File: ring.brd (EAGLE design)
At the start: 174.9 x 190 mm, 36 parts

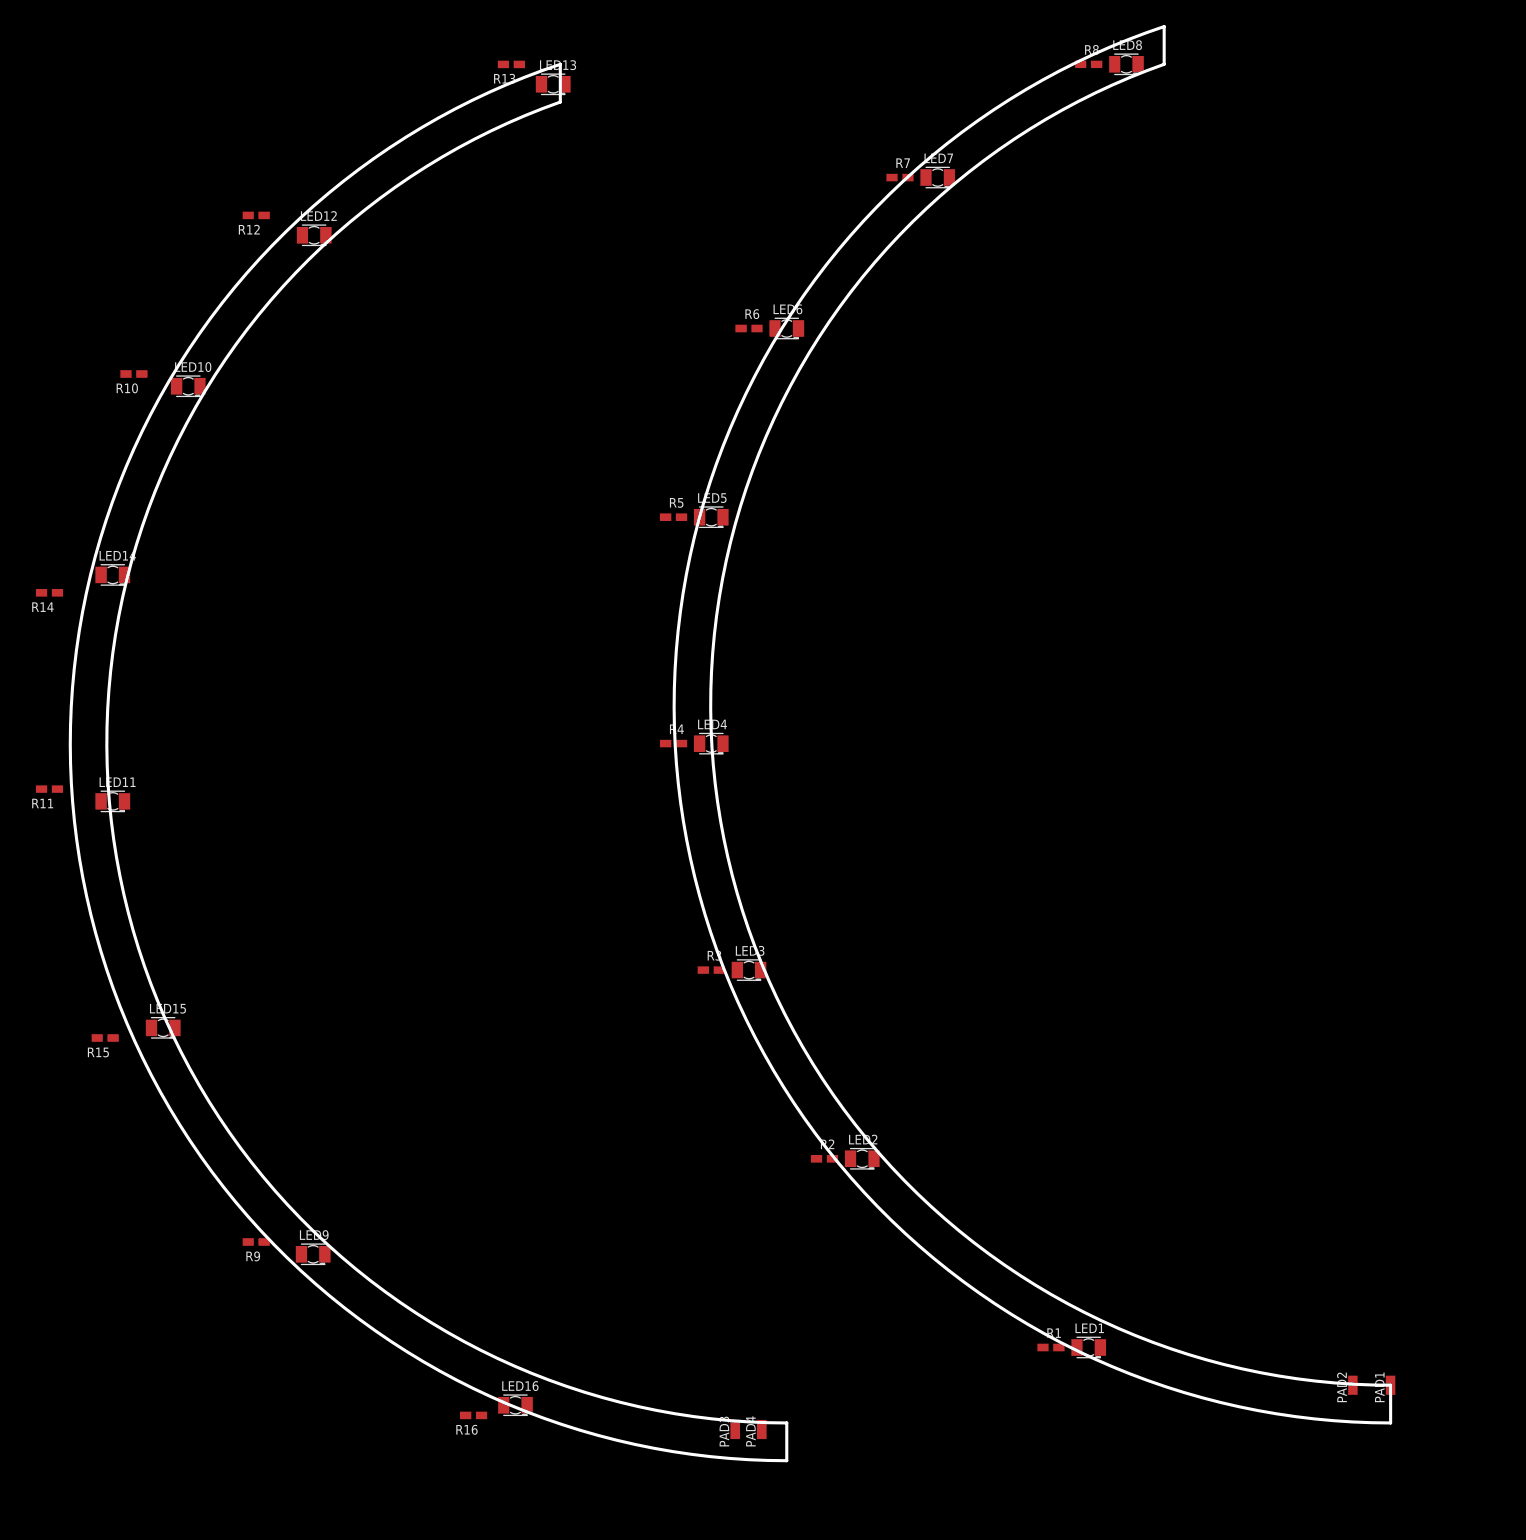
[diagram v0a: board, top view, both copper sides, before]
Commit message: polygon
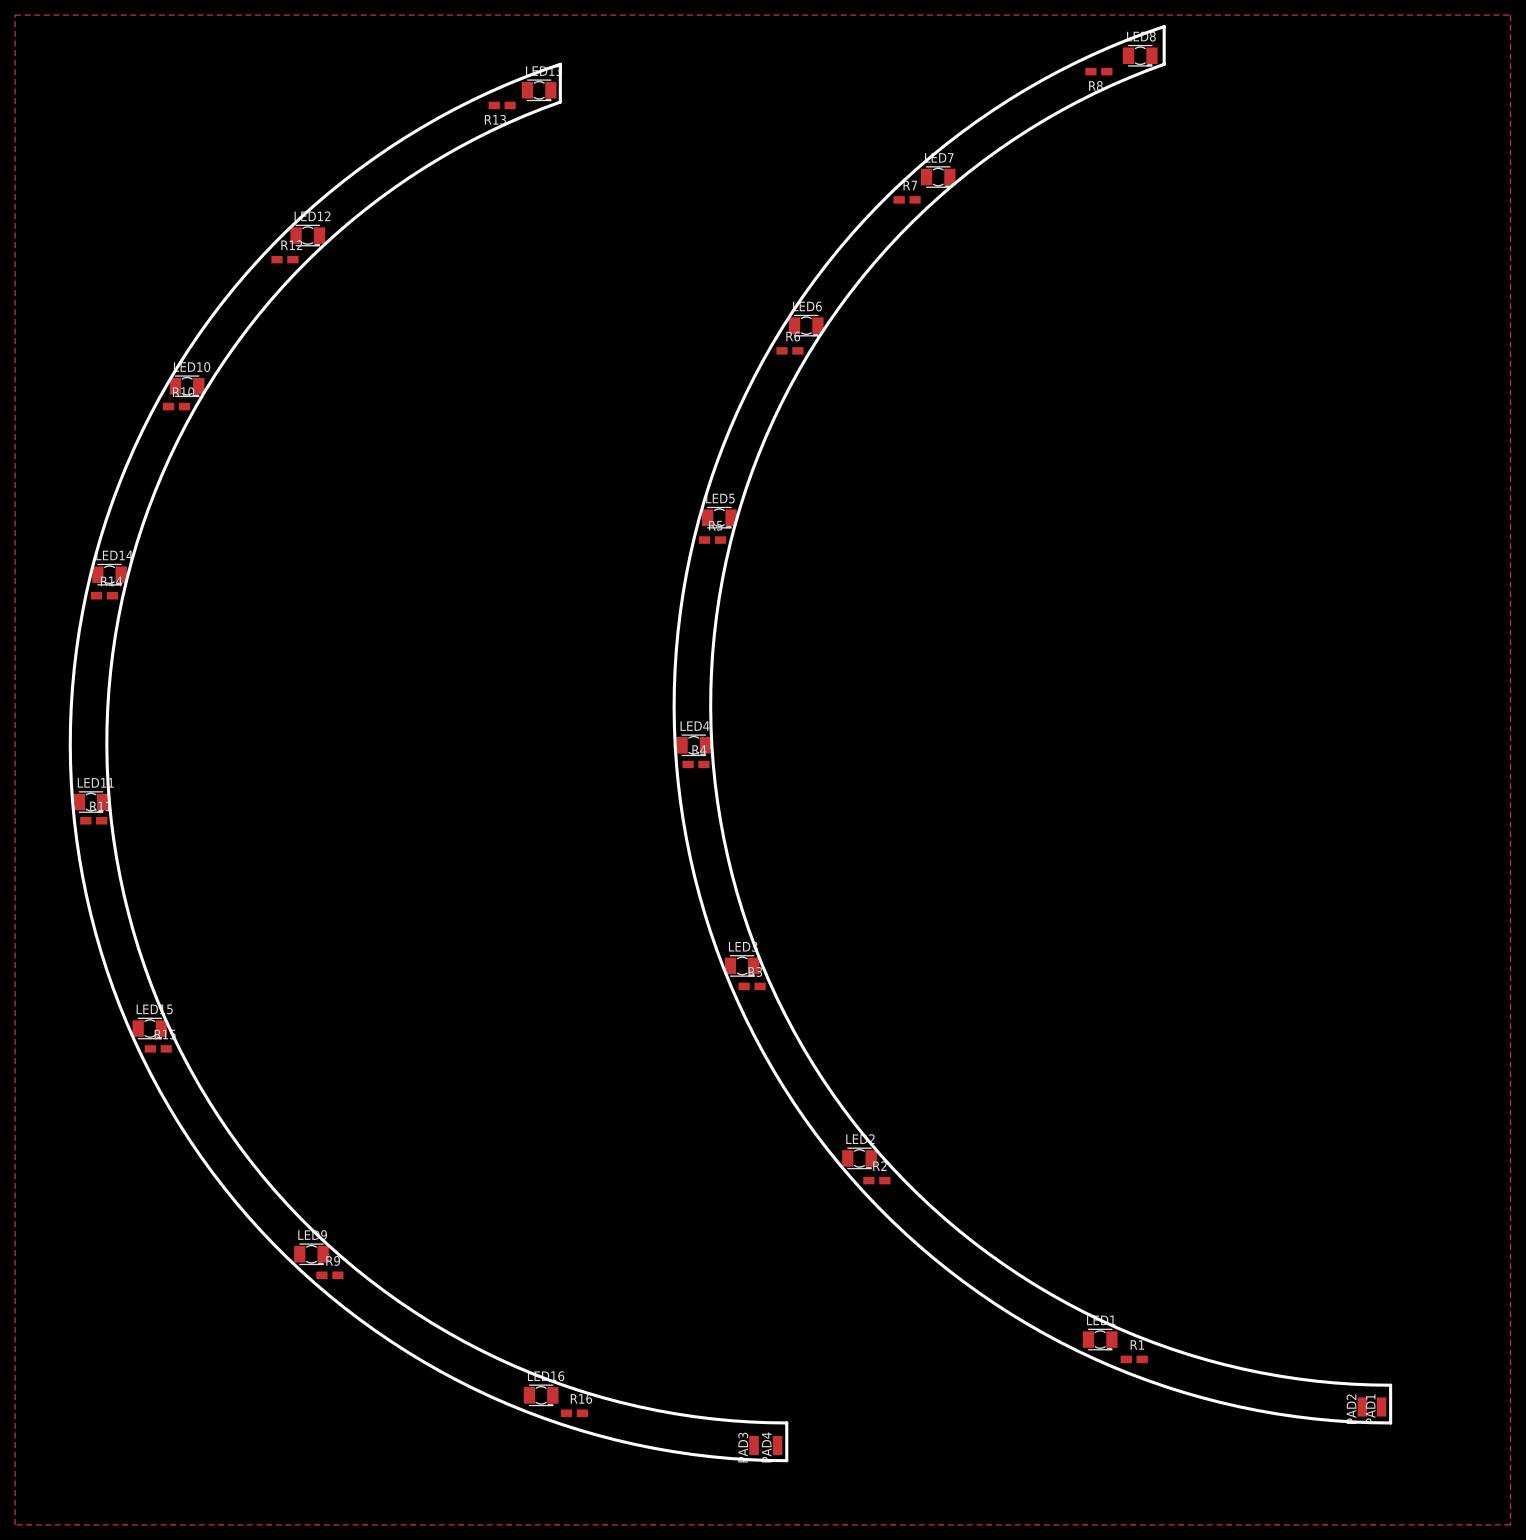
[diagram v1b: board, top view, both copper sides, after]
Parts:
- moved R16 13.4 mm to (-28.1, -88.7), turned to 0 degrees
- moved R1 11.1 mm to (46.0, -81.6)
- moved R9 10.7 mm to (-60.5, -70.4), turned to 0 degrees
- moved R2 7.52 mm to (11.9, -57.9)
- moved R14 7.29 mm to (-90.4, 19.6), turned to 0 degrees
- moved R11 7.21 mm to (-91.8, -10.2), turned to 0 degrees
- moved R15 7.18 mm to (-83.3, -40.4), turned to 0 degrees
- moved R10 7.10 mm to (-80.8, 44.7), turned to 0 degrees
- moved R12 7.00 mm to (-66.5, 64.1), turned to 0 degrees
- moved R6 6.18 mm to (0.42, 52.0)
- moved R5 5.99 mm to (-9.83, 27.0)
- moved R3 5.83 mm to (-4.59, -32.2)
- moved R13 5.58 mm to (-37.7, 84.5)
- moved R4 4.06 mm to (-12.0, -2.76)
- moved LED16 3.65 mm to (-32.5, -86.3)
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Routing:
- added copper zone on layer 1, net GND

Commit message: nentime
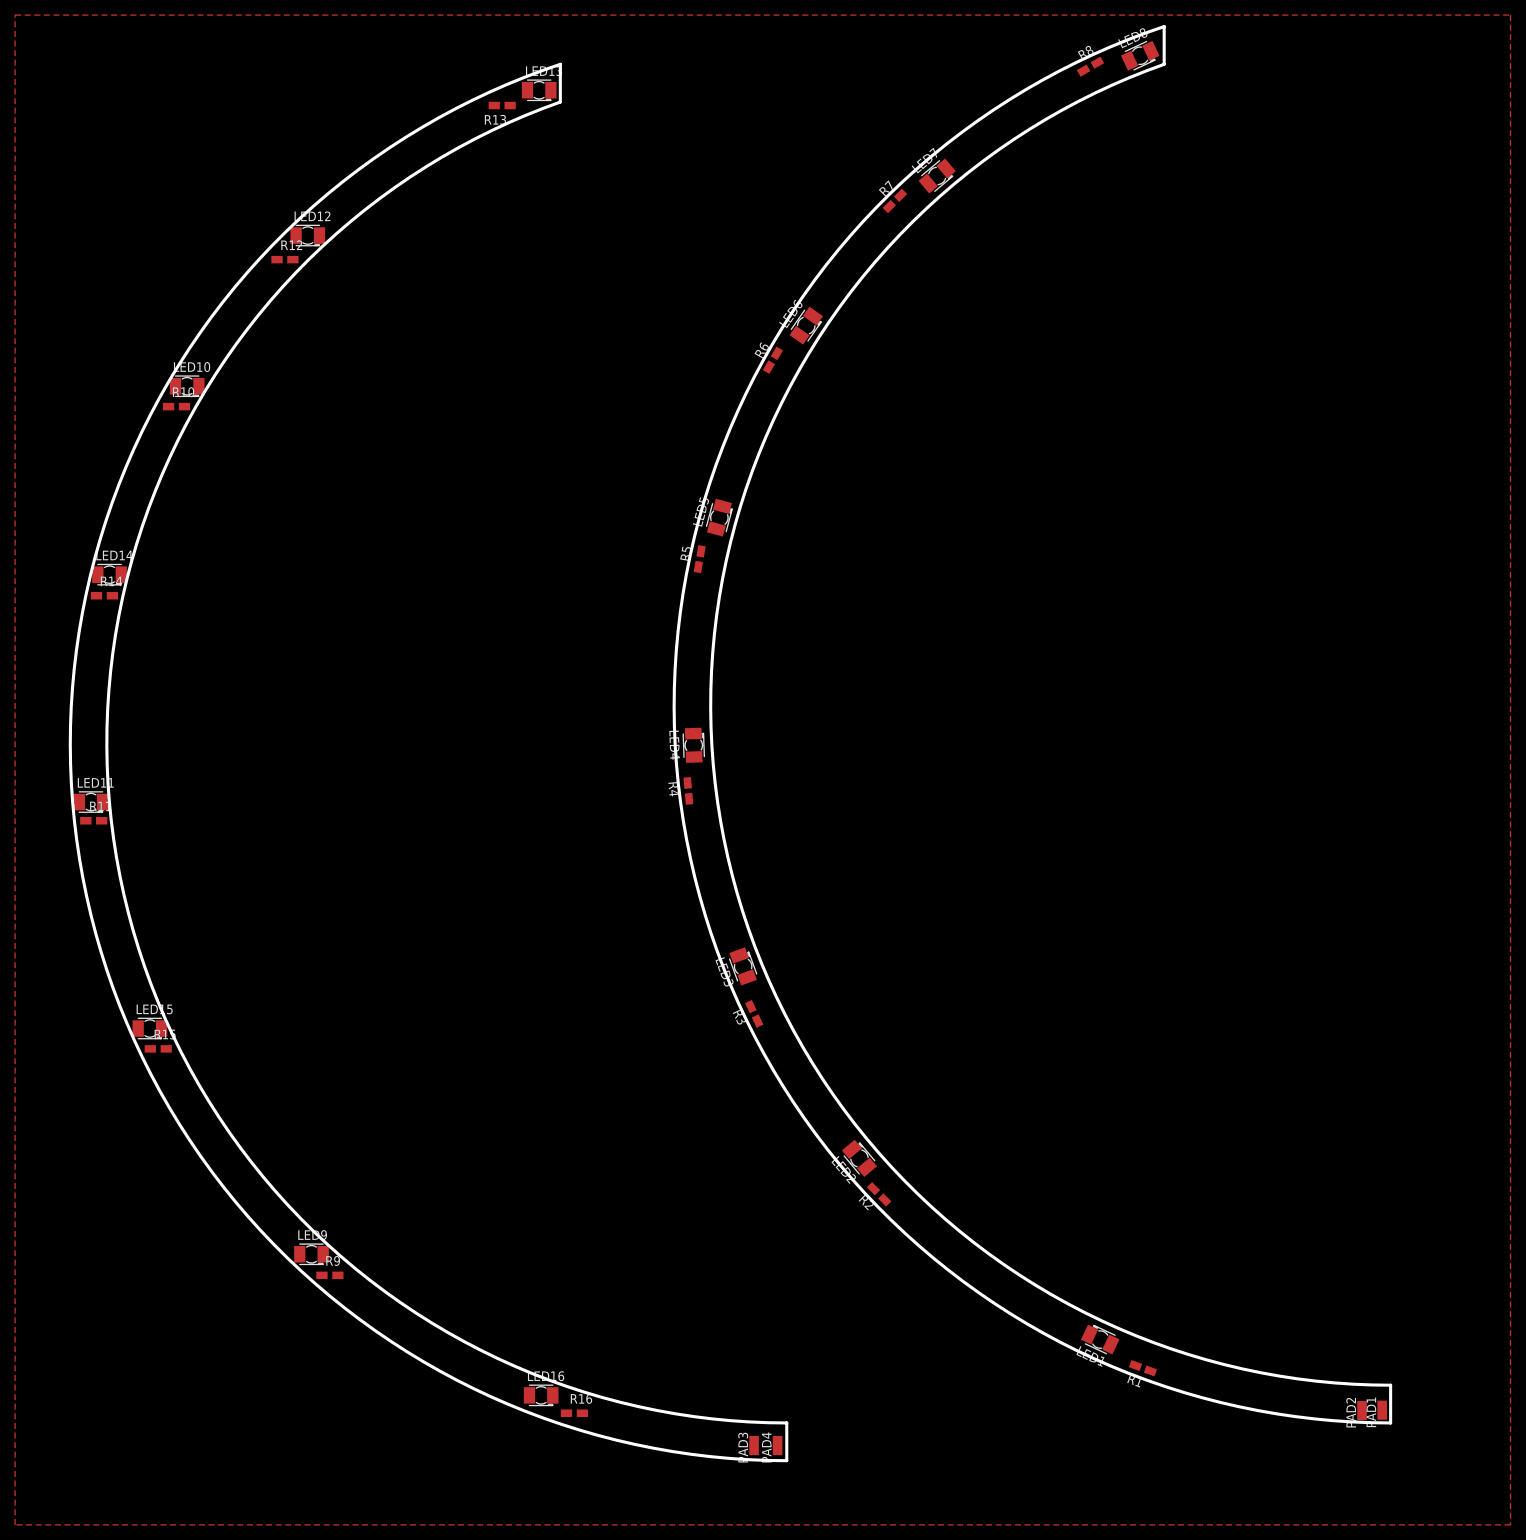
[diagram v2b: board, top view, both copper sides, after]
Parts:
- moved R3 3.65 mm to (-4.31, -35.8), turned to 115 degrees
- moved R4 3.65 mm to (-13.0, -6.26), turned to 95 degrees
- moved R5 3.05 mm to (-11.5, 24.4), turned to 80 degrees
- moved R6 2.58 mm to (-1.84, 50.8), turned to 60 degrees
- moved R2 1.84 mm to (12.2, -59.7), turned to 135 degrees
- moved R1 1.65 mm to (47.2, -82.8), turned to 160 degrees
- moved R7 1.62 mm to (14.3, 71.9), turned to 45 degrees
- moved R8 1.28 mm to (40.2, 89.7), turned to 30 degrees
- moved PAD2 0.46 mm to (76.2, -88.4)
- moved PAD1 0.42 mm to (78.9, -88.3)
- moved LED7 0.20 mm to (19.9, 75.2), turned to 40 degrees
- moved LED3 0.15 mm to (-5.78, -29.5), turned to 110 degrees
- turned LED1 to 155 degrees
- turned LED2 to 130 degrees
- turned LED4 to 92 degrees
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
